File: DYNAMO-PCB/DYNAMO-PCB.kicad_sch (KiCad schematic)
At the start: 13 parts, among them J13 Conn_01x02_Pin, J14 Conn_01x05_Pin, J18 USB3_A, J21 USB3_A, J22 USB3_A, J23 USB3_A, J24 USB3_A, J25 USB3_A, J3 Conn_01x03_Pin, J4 Conn_01x05_Pin

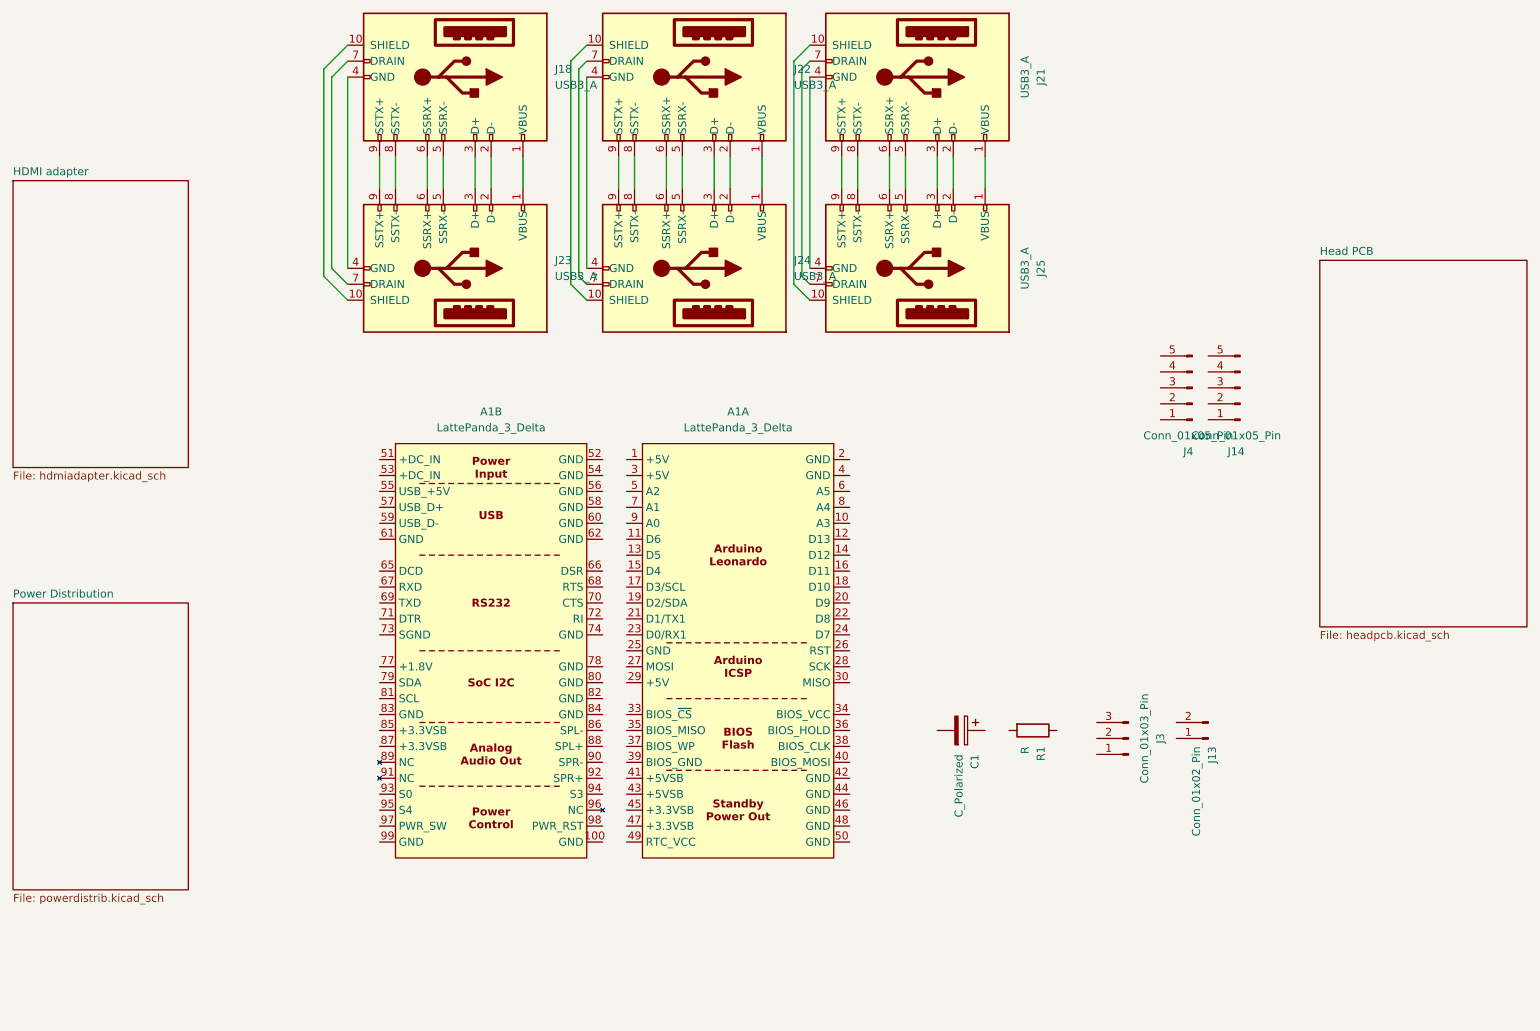
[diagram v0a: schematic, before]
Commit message: schematic wip
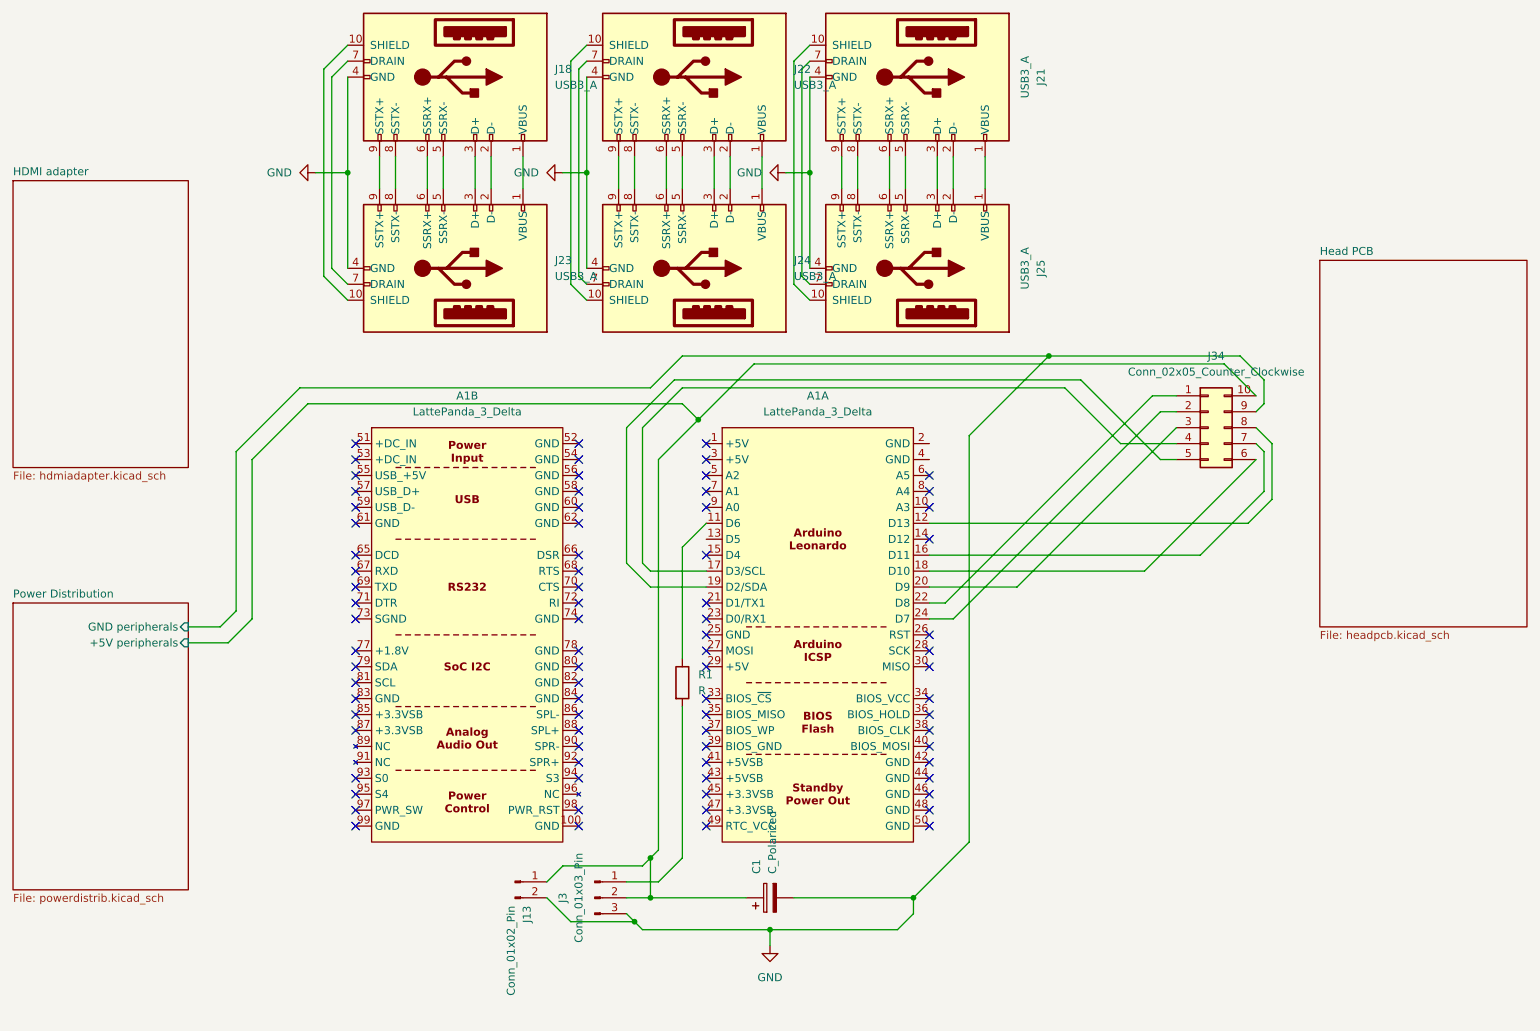
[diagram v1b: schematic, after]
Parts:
- removed J14, J4: Conn_01x05_Pin, Connector_PinHeader_2.54mm:PinHeader_1x05_P2.54mm_Vertical, symbol Connector:Conn_01x05_Pin
- added J34: Conn_02x05_Counter_Clockwise, Connector_PinHeader_2.54mm:PinHeader_2x05_P2.54mm_Vertical, symbol Connector_Generic:Conn_02x05_Counter_Clockwise
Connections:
- net GND: now reaches J22.4 (GND), J24.4 (GND)
- net GND: now also C1.2, J13.2 (Pin_2), J18.4 (GND), J21.4 (GND), J23.4 (GND), J25.4 (GND), J3.3 (Pin_3), J34.9 (Pin_9)
- net at J3.1 (Pin_1): now also R1.2
- net Power Distribution/+5V peripherals: now reaches J3.2 (Pin_2)
- net Power Distribution/+5V peripherals: now also C1.1, J13.1 (Pin_1), J34.10 (Pin_10)
- net at A1.11 (D6): now also R1.1
- net at A1.12 (D13): now also J34.8 (Pin_8)
- net at A1.16 (D11): now also J34.7 (Pin_7)
- net at A1.17 (D3/SCL): now also J34.4 (Pin_4)
- net at A1.18 (D10): now also J34.6 (Pin_6)
- net at A1.19 (D2/SDA): now also J34.5 (Pin_5)
- net at A1.20 (D9): now also J34.3 (Pin_3)
- net at A1.22 (D8): now also J34.1 (Pin_1)
- net at A1.24 (D7): now also J34.2 (Pin_2)
- no-connect marks 0 -> 79
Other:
- sheet Power Distribution ports: added +5V peripherals, GND peripherals; removed none
- moved on the sheet: A1A, A1B, C1, J13, J3, R1

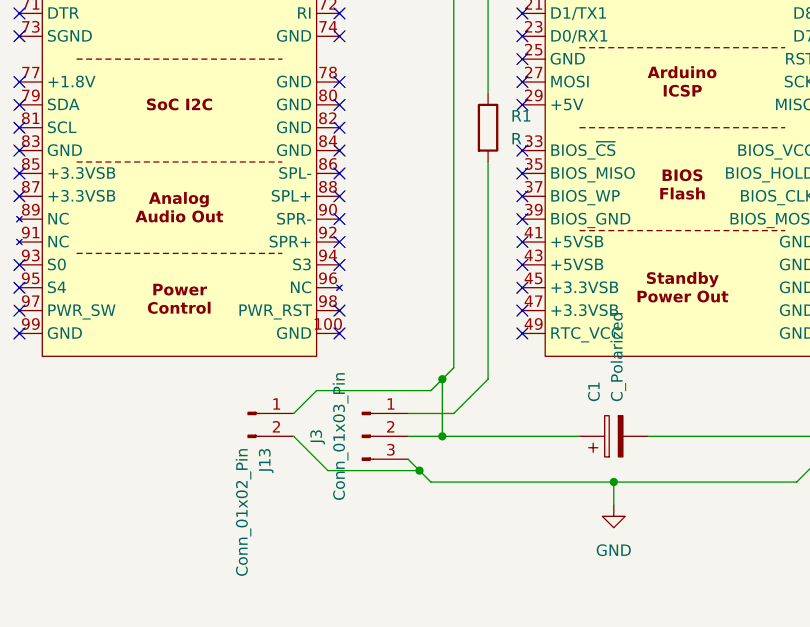
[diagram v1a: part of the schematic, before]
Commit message: schematic wip
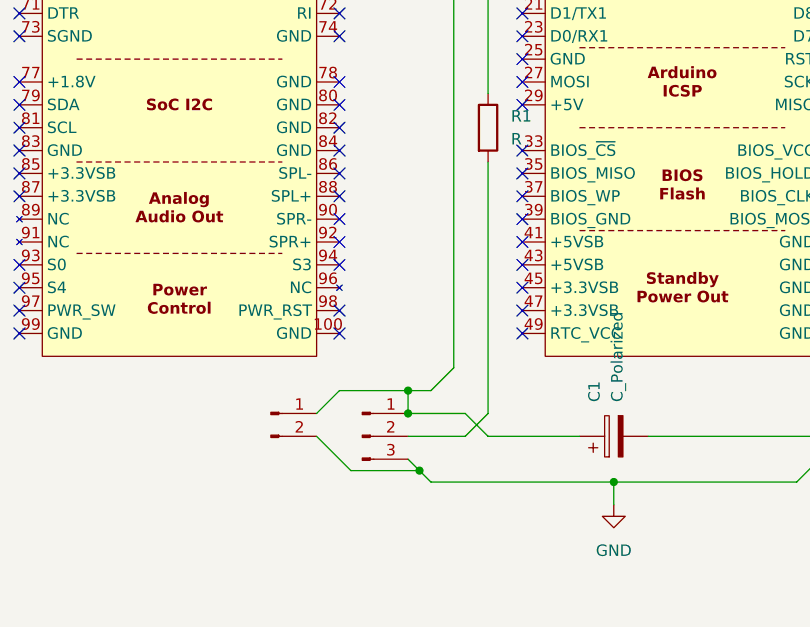
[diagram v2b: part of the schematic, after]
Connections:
- net Power Distribution/+5V peripherals: now also J3.1 (Pin_1); no longer J3.2 (Pin_2)
- net at R1.2: now also J3.2 (Pin_2); no longer J3.1 (Pin_1)
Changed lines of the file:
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@@
 	(paper "A4")
 	(junction
-		(at 132.08 156.21)
+		(at 128.27 157.48)
 		(diameter 0)
 		(color 0 0 0 0)
@@
 	)
 	(junction
-		(at 132.08 162.56)
-		(diameter 0)
-		(color 0 0 0 0)
-	)
-	(junction
 		(at 173.99 162.56)
 		(diameter 0)
@@
 	)
 	(junction
+		(at 128.27 160.02)
+		(diameter 0)
+		(color 0 0 0 0)
+	)
+	(junction
 		(at 151.13 167.64)
 		(diameter 0)
@@
 	(wire
 		(pts
-			(xy 128.27 160.02) (xy 133.35 160.02)
-		)
-		(stroke
-			(width 0)
-			(type default)
-		)
-	)
-	(wire
-		(pts
 			(xy 229.87 91.44) (xy 228.6 90.17)
 		)
@@
 	(wire
 		(pts
+			(xy 147.32 162.56) (xy 137.16 162.56)
+		)
+		(stroke
+			(width 0)
+			(type default)
+		)
+	)
+	(wire
+		(pts
 			(xy 83.82 67.31) (xy 80.01 63.5)
 		)
@@
 	(wire
 		(pts
-			(xy 132.08 156.21) (xy 133.35 154.94)
+			(xy 130.81 157.48) (xy 133.35 154.94)
 		)
 		(stroke
@@
 	(wire
 		(pts
-			(xy 133.35 160.02) (xy 137.16 156.21)
-		)
-		(stroke
-			(width 0)
-			(type default)
-		)
-	)
-	(wire
-		(pts
 			(xy 157.48 67.31) (xy 154.94 64.77)
 		)
@@
 	(wire
 		(pts
-			(xy 132.08 162.56) (xy 147.32 162.56)
-		)
-		(stroke
-			(width 0)
-			(type default)
-		)
-	)
-	(wire
-		(pts
 			(xy 129.54 44.45) (xy 129.54 49.53)
 		)
@@
 	(wire
 		(pts
+			(xy 137.16 162.56) (xy 134.62 160.02)
+		)
+		(stroke
+			(width 0)
+			(type default)
+		)
+	)
+	(wire
+		(pts
 			(xy 132.08 110.49) (xy 130.81 109.22)
 		)
@@
 	(wire
 		(pts
-			(xy 129.54 166.37) (xy 119.38 166.37)
+			(xy 137.16 132.08) (xy 137.16 160.02)
+		)
+		(stroke
+			(width 0)
+			(type default)
+		)
+	)
+	(wire
+		(pts
+			(xy 129.54 166.37) (xy 121.92 166.37)
 		)
 		(stroke
@@
 	(wire
 		(pts
-			(xy 132.08 156.21) (xy 132.08 162.56)
-		)
-		(stroke
-			(width 0)
-			(type default)
-		)
-	)
-	(wire
-		(pts
 			(xy 213.36 92.71) (xy 215.9 92.71)
 		)
@@
 	(wire
 		(pts
+			(xy 128.27 162.56) (xy 134.62 162.56)
+		)
+		(stroke
+			(width 0)
+			(type default)
+		)
+	)
+	(wire
+		(pts
 			(xy 200.66 80.01) (xy 213.36 92.71)
 		)
@@
 	(wire
 		(pts
-			(xy 130.81 157.48) (xy 132.08 156.21)
-		)
-		(stroke
-			(width 0)
-			(type default)
-		)
-	)
-	(wire
-		(pts
 			(xy 80.01 63.5) (xy 80.01 30.48)
 		)
@@
 	(wire
 		(pts
+			(xy 128.27 157.48) (xy 120.65 157.48)
+		)
+		(stroke
+			(width 0)
+			(type default)
+		)
+	)
+	(wire
+		(pts
 			(xy 229.87 83.82) (xy 228.6 85.09)
 		)
@@
 	(wire
 		(pts
-			(xy 137.16 132.08) (xy 137.16 156.21)
-		)
-		(stroke
-			(width 0)
-			(type default)
-		)
-	)
-	(wire
-		(pts
-			(xy 128.27 162.56) (xy 132.08 162.56)
-		)
-		(stroke
-			(width 0)
-			(type default)
-		)
-	)
-	(wire
-		(pts
 			(xy 180.34 118.11) (xy 213.36 85.09)
 		)
@@
 	(wire
 		(pts
-			(xy 130.81 157.48) (xy 118.11 157.48)
+			(xy 130.81 157.48) (xy 128.27 157.48)
 		)
 		(stroke
@@
 	(wire
 		(pts
+			(xy 128.27 160.02) (xy 134.62 160.02)
+		)
+		(stroke
+			(width 0)
+			(type default)
+		)
+	)
+	(wire
+		(pts
 			(xy 118.11 46.99) (xy 121.92 46.99)
 		)
@@
 	(wire
 		(pts
-			(xy 119.38 166.37) (xy 115.57 162.56)
+			(xy 121.92 166.37) (xy 118.11 162.56)
 		)
 		(stroke
@@
 	(wire
 		(pts
-			(xy 118.11 157.48) (xy 115.57 160.02)
+			(xy 120.65 157.48) (xy 118.11 160.02)
 		)
 		(stroke
@@
 	(wire
 		(pts
+			(xy 128.27 157.48) (xy 128.27 160.02)
+		)
+		(stroke
+			(width 0)
+			(type default)
+		)
+	)
+	(wire
+		(pts
 			(xy 81.28 31.75) (xy 83.82 29.21)
+		)
+		(stroke
+			(width 0)
+			(type default)
+		)
+	)
+	(wire
+		(pts
+			(xy 137.16 160.02) (xy 134.62 162.56)
 		)
 		(stroke
@@
 					(size 1.27 1.27)
 				)
+				(hide yes)
 			)
 		)
@@
 					(size 1.27 1.27)
 				)
+				(hide yes)
 			)
 		)
@@
 	(symbol
 		(lib_id "Connector:Conn_01x02_Pin")
-		(at 110.49 160.02 0)
+		(at 113.03 160.02 0)
 		(unit 1)
 		(exclude_from_sim no)
@@
 		(dnp no)
 		(property "Reference" "J13"
+			(at 114.9351 163.83 90)
+			(effects
+				(font
+					(size 1.27 1.27)
+				)
+				(justify right)
+				(hide yes)
+			)
+		)
+		(property "Value" "Conn_01x02_Pin"
 			(at 112.3951 163.83 90)
 			(effects
@@
 				)
 				(justify right)
-			)
-		)
-		(property "Value" "Conn_01x02_Pin"
-			(at 109.8551 163.83 90)
-			(effects
-				(font
-					(size 1.27 1.27)
-				)
-				(justify right)
+				(hide yes)
 			)
 		)
 		(property "Footprint" "Connector_PinHeader_2.54mm:PinHeader_1x02_P2.54mm_Vertical"
-			(at 110.49 160.02 0)
+			(at 113.03 160.02 0)
 			(effects
 				(font
@@
 		)
 		(property "Datasheet" "~"
-			(at 110.49 160.02 0)
+			(at 113.03 160.02 0)
 			(effects
 				(font
@@
 		)
 		(property "Description" "Generic connector, single row, 01x02, script generated"
-			(at 110.49 160.02 0)
-			(effects
-				(font
+			(at 113.03 160.02 0)
+			(effects
+				(font
